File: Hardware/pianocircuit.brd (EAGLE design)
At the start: 160 x 100 mm, 70 parts, among them IC1 LM386M-1

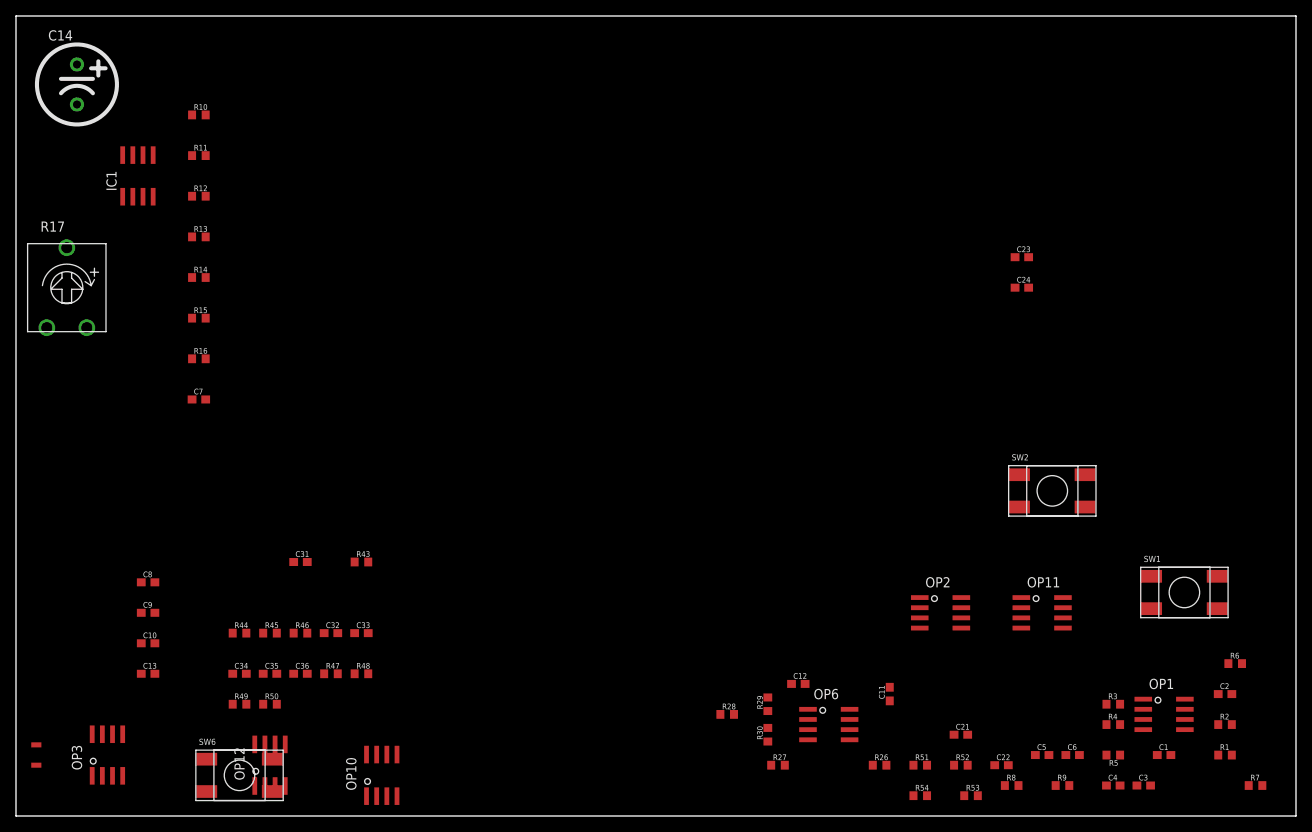
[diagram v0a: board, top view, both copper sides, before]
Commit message: Board Routing
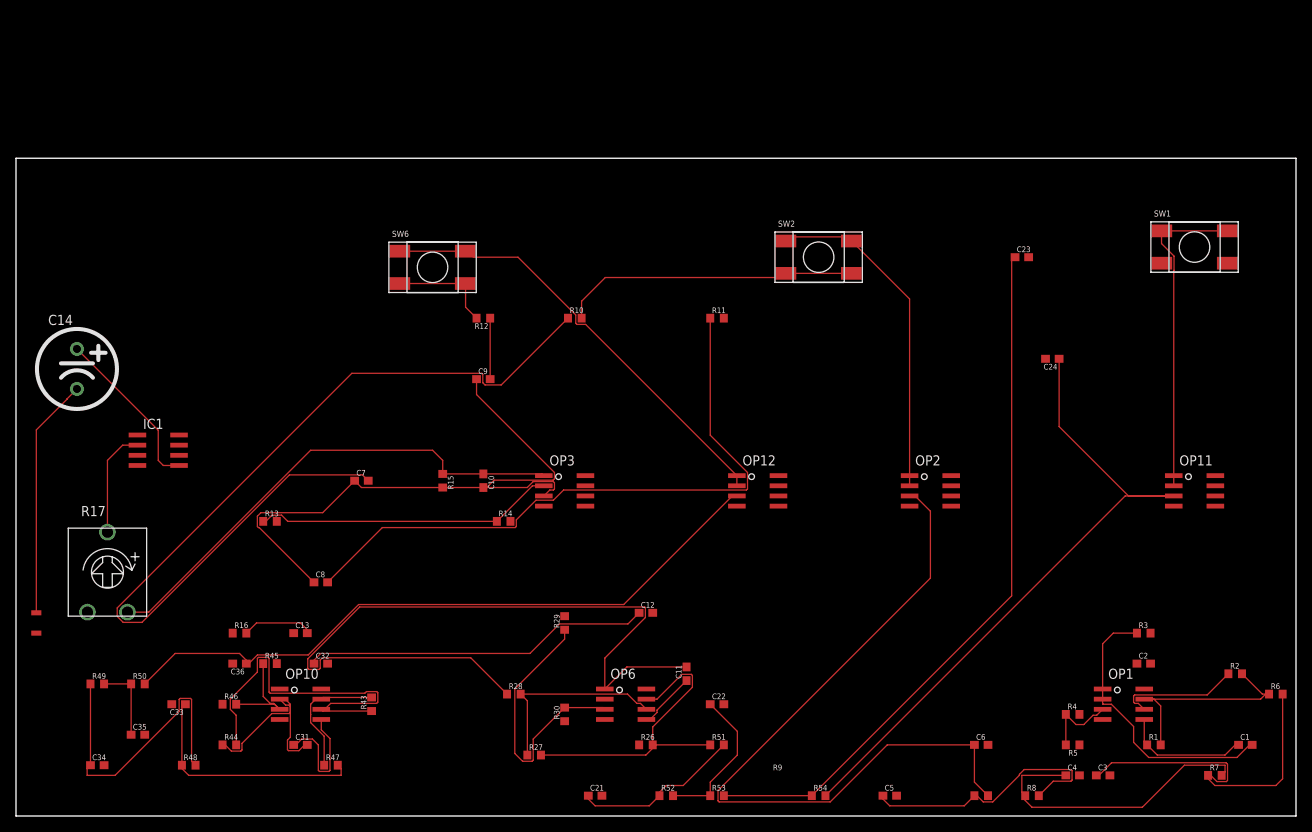
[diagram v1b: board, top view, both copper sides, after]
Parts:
- moved OP12 69.9 mm to (92.7, 40.6), turned to 270 degrees
- moved SW6 67.9 mm to (52.1, 68.6)
- moved R11 67.9 mm to (87.6, 62.2)
- moved OP3 66.0 mm to (68.6, 40.6), turned to 270 degrees
- moved R10 53.4 mm to (69.8, 62.2)
- moved C9 51.1 mm to (58.4, 54.6)
- moved R14 48.8 mm to (61.0, 36.8)
- moved C10 46.6 mm to (58.4, 41.9), turned to 270 degrees
- moved C21 46.4 mm to (72.4, 2.54)
- moved SW1 43.2 mm to (147.3, 71.1)
- moved SW2 41.3 mm to (100.3, 69.8)
- moved R12 38.7 mm to (58.4, 62.2), turned to 180 degrees
- moved R52 37.0 mm to (81.3, 2.54)
- moved R13 36.7 mm to (31.8, 36.8)
- moved R15 36.6 mm to (53.3, 41.9), turned to 270 degrees
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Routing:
- net N$14: track 0.00 -> 113.9 mm
- net N$28: track 0.00 -> 97.8 mm
- net N$10: track 0.00 -> 92.7 mm
- net N$54: track 0.00 -> 88.8 mm
- net N$55: track 0.00 -> 85.5 mm
- net N$65: track 0.00 -> 85.1 mm
- net N$17: track 0.00 -> 81.1 mm
- net N$15: track 0.00 -> 79.9 mm
- net N$20: track 0.00 -> 62.7 mm
- net N$66: track 0.00 -> 54.4 mm
- net N$58: track 0.00 -> 47.0 mm
- net N$2: track 0.00 -> 43.5 mm
- net N$11: track 0.00 -> 43.0 mm
- net N$7: track 0.00 -> 43.0 mm
- net N$57: track 0.00 -> 40.7 mm
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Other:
- board size 160 x 100 mm -> 160 x 82.2 mm
